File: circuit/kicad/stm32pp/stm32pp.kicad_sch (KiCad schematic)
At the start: 33 parts, among them J1 USB_B_Micro, J2 USB_B_Micro, J3 Conn_01x04_Male, J4 Conn_01x08_Male, J5 Conn_01x08_Male, J6 Conn_01x08_Male, J7 Conn_01x08_Male, SW1 SW_Push, SW2 SW_Push, SW3 SW_Push, U1 STM32F103C8Tx, U2 CH340C, U3 AMS1117-3.3

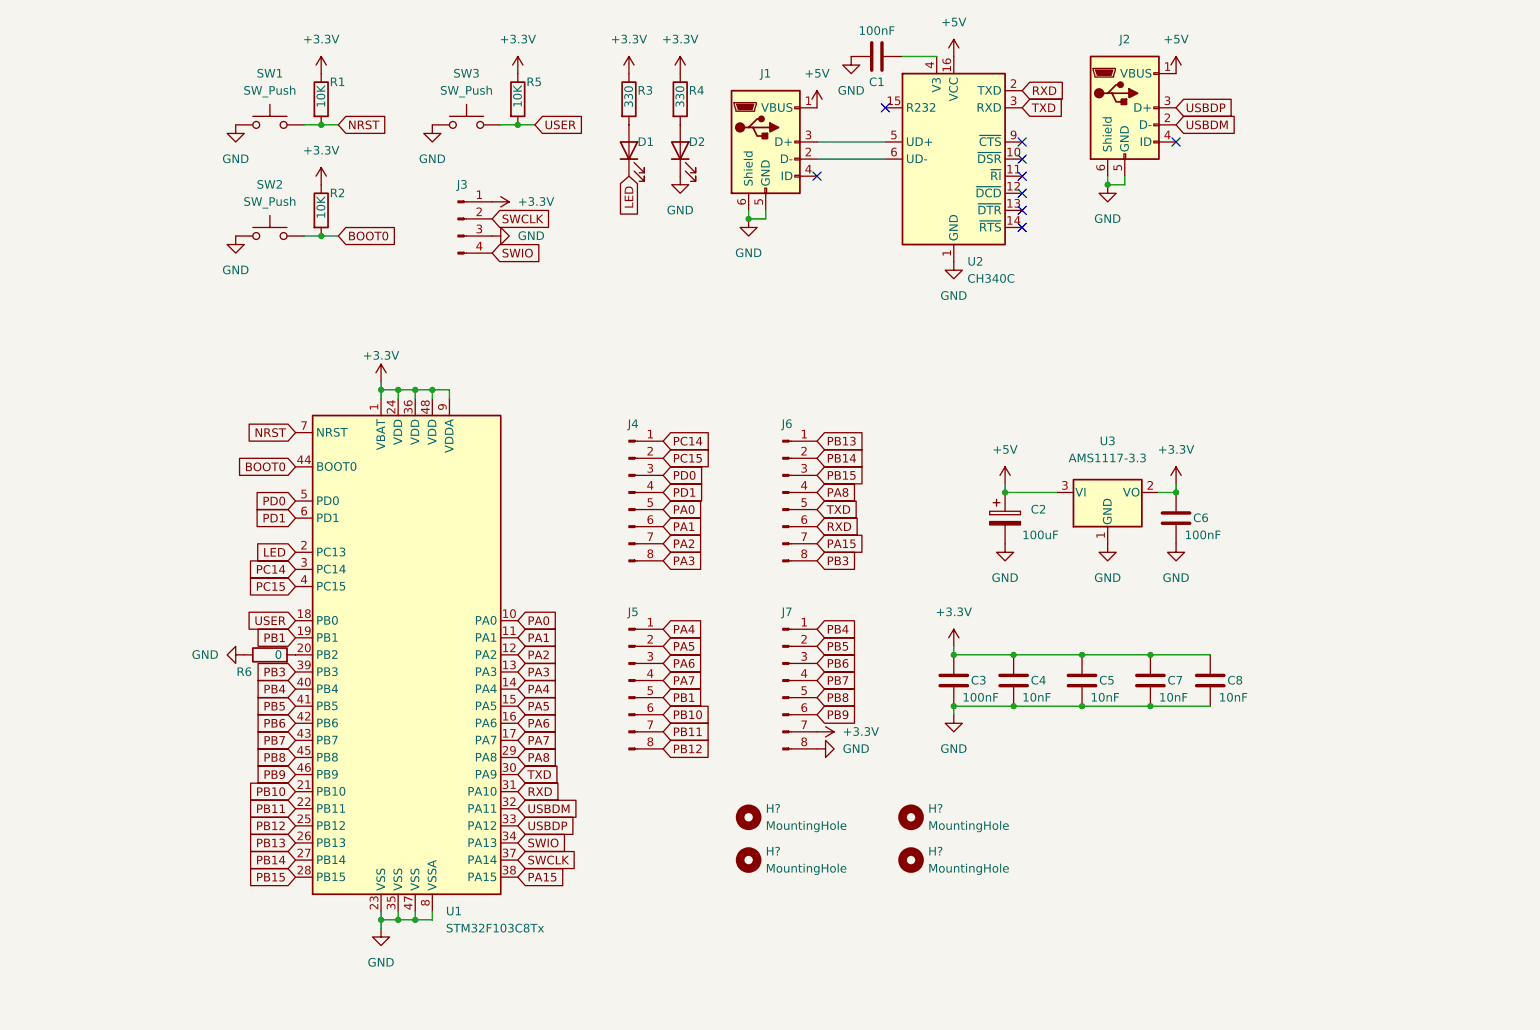
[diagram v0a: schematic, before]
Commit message: STM32PP
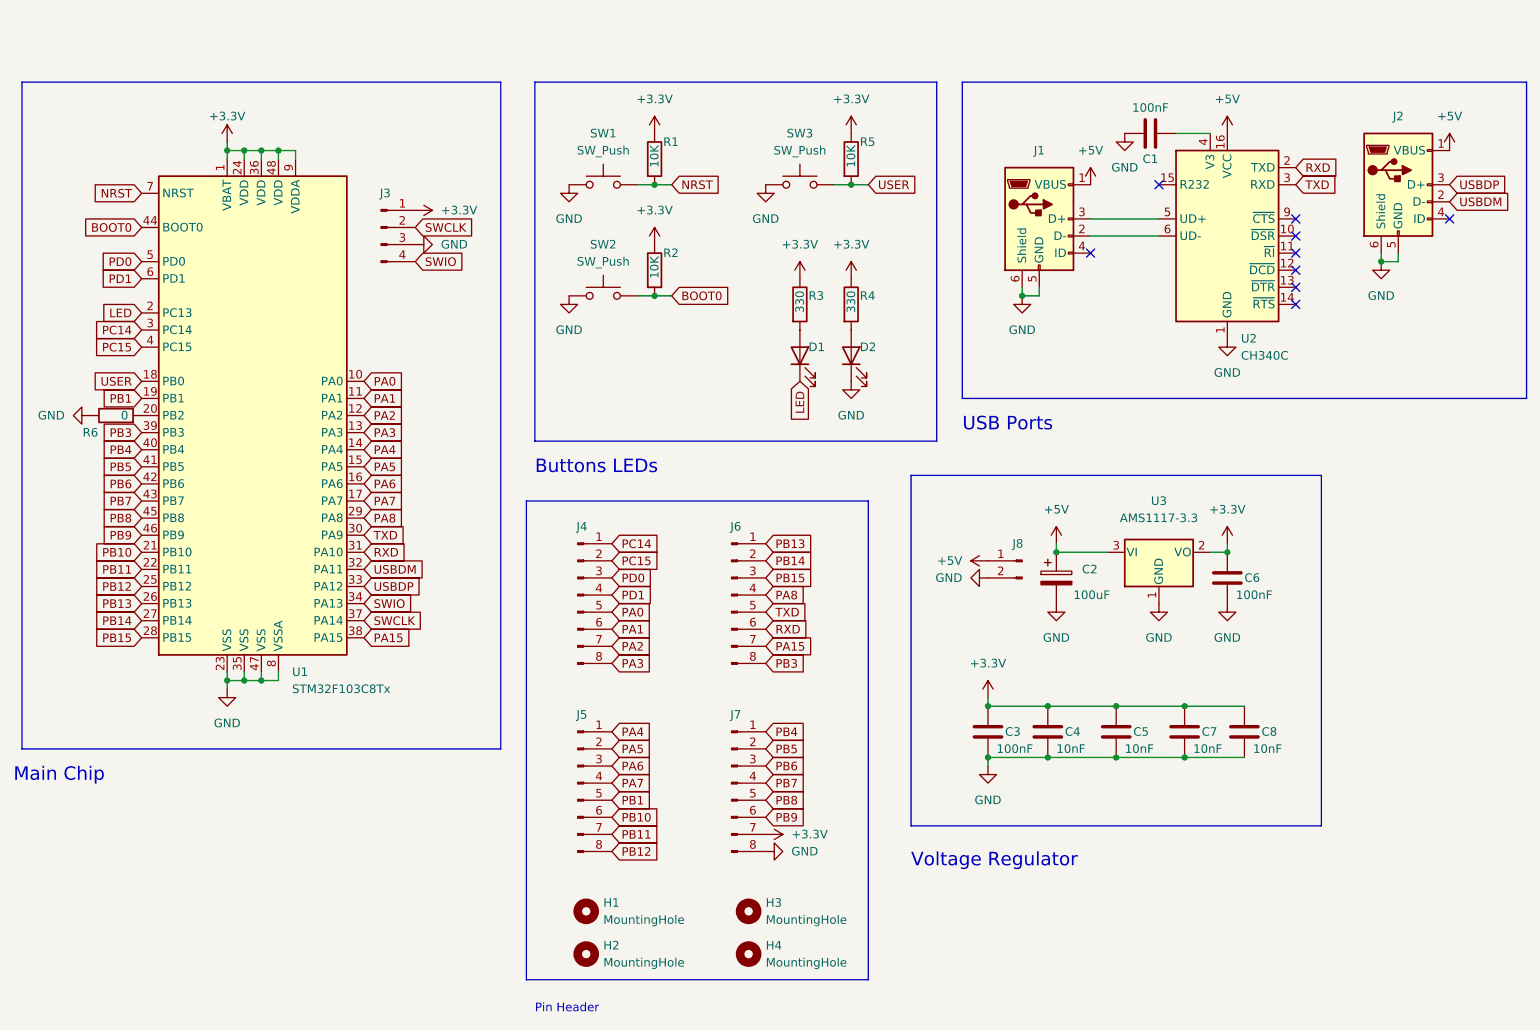
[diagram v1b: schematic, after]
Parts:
- added J8: Conn_01x02_Male, symbol Connector:Conn_01x02_Male
- gave numbers to parts that had none: 4
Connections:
- net +5V: now also J8.1 (Pin_1)
- net GND: now also J8.2 (Pin_2)
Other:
- note added: "Buttons LEDs"
- note added: "Main Chip"
- note added: "Pin Header"
- note added: "USB Ports"
- note added: "Voltage Regulator"
- moved on the sheet: C1, C2, C3, C4, C5, C6, C7, C8, D1, D2, H1, H2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
